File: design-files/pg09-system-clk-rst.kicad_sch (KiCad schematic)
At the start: 16 parts, among them J201 Clock Source, J202 Reset Connector, Q201 2N7000, SW201 SW_Push, U201 CD74ACT109, U202 CD74ACT163, U203 DS1813, X201 ACO-32.000MHz

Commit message: Assign a bunch of footprints.
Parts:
- C201, C202, C203: footprint (none) -> Capacitor_THT:C_Disc_D6.0mm_W4.4mm_P5.00mm
- U201, U202: footprint (none) -> Package_DIP:DIP-16_W7.62mm_Socket
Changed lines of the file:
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@@
       (effects (font (size 1.27 1.27)) (justify left))
     )
-    (property "Footprint" "" (at 196.215 79.375 0)
+    (property "Footprint" "Package_DIP:DIP-16_W7.62mm_Socket" (at 196.215 79.375 0)
       (effects (font (size 1.27 1.27)) hide)
     )
@@
       (effects (font (size 1.27 1.27)) (justify left))
     )
-    (property "Footprint" "" (at 214.63 110.49 0)
+    (property "Footprint" "Capacitor_THT:C_Disc_D6.0mm_W4.4mm_P5.00mm" (at 214.63 110.49 0)
       (effects (font (size 1.27 1.27)) hide)
     )
@@
       (effects (font (size 1.27 1.27)) (justify left))
     )
-    (property "Footprint" "" (at 204.47 110.49 0)
+    (property "Footprint" "Capacitor_THT:C_Disc_D6.0mm_W4.4mm_P5.00mm" (at 204.47 110.49 0)
       (effects (font (size 1.27 1.27)) hide)
     )
@@
       (effects (font (size 1.27 1.27)) (justify left))
     )
-    (property "Footprint" "" (at 194.31 110.49 0)
+    (property "Footprint" "Capacitor_THT:C_Disc_D6.0mm_W4.4mm_P5.00mm" (at 194.31 110.49 0)
       (effects (font (size 1.27 1.27)) hide)
     )
@@
       (effects (font (size 1.27 1.27)) (justify left))
     )
-    (property "Footprint" "" (at 169.545 111.125 0)
+    (property "Footprint" "Package_DIP:DIP-16_W7.62mm_Socket" (at 169.545 111.125 0)
       (effects (font (size 1.27 1.27)) hide)
     )
@@
       (effects (font (size 1.27 1.27)) (justify left))
     )
-    (property "Footprint" "" (at 169.545 79.375 0)
+    (property "Footprint" "Package_DIP:DIP-16_W7.62mm_Socket" (at 169.545 79.375 0)
       (effects (font (size 1.27 1.27)) hide)
     )
@@
       (effects (font (size 1.27 1.27)) (justify left))
     )
-    (property "Footprint" "" (at 95.885 89.535 0)
-      (effects (font (size 1.27 1.27)) hide)
-    )
+    (property "Footprint" "Package_DIP:DIP-16_W7.62mm_Socket" (at 95.885 89.535 0)
+      (effects (font (size 1.27 1.27)) hide)
+    )

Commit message: Finish assigning footprints.
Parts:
- R201, R202, R203, R204, R205: footprint (none) -> Resistor_THT:R_Axial_DIN0207_L6.3mm_D2.5mm_P7.62mm_Horizontal
- SW201: footprint (none) -> Button_Switch_THT:SW_PUSH_6mm
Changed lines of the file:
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@@
       (effects (font (size 1.27 1.27)) (justify left))
     )
-    (property "Footprint" "" (at 220.345 76.835 0)
+    (property "Footprint" "Resistor_THT:R_Axial_DIN0207_L6.3mm_D2.5mm_P7.62mm_Horizontal" (at 220.345 76.835 0)
       (effects (font (size 1.27 1.27)) hide)
     )
@@
       (effects (font (size 1.27 1.27)) (justify right))
     )
-    (property "Footprint" "" (at 212.725 88.265 0)
+    (property "Footprint" "Resistor_THT:R_Axial_DIN0207_L6.3mm_D2.5mm_P7.62mm_Horizontal" (at 212.725 88.265 0)
       (effects (font (size 1.27 1.27)) hide)
     )
@@
       (effects (font (size 1.27 1.27)))
     )
-    (property "Footprint" "" (at 100.965 163.195 0)
+    (property "Footprint" "Button_Switch_THT:SW_PUSH_6mm" (at 100.965 163.195 0)
       (effects (font (size 1.27 1.27)) hide)
     )
@@
       (effects (font (size 1.27 1.27)) (justify right))
     )
-    (property "Footprint" "" (at 84.455 151.765 0)
+    (property "Footprint" "Resistor_THT:R_Axial_DIN0207_L6.3mm_D2.5mm_P7.62mm_Horizontal" (at 84.455 151.765 0)
       (effects (font (size 1.27 1.27)) hide)
     )
@@
       (effects (font (size 1.27 1.27)))
     )
-    (property "Footprint" "" (at 219.075 59.69 0)
+    (property "Footprint" "Resistor_THT:R_Axial_DIN0207_L6.3mm_D2.5mm_P7.62mm_Horizontal" (at 219.075 59.69 0)
       (effects (font (size 1.27 1.27)) hide)
     )
@@
       (effects (font (size 1.27 1.27)))
     )
-    (property "Footprint" "" (at 219.075 66.675 0)
-      (effects (font (size 1.27 1.27)) hide)
-    )
+    (property "Footprint" "Resistor_THT:R_Axial_DIN0207_L6.3mm_D2.5mm_P7.62mm_Horizontal" (at 219.075 66.675 0)
+      (effects (font (size 1.27 1.27)) hide)
+    )

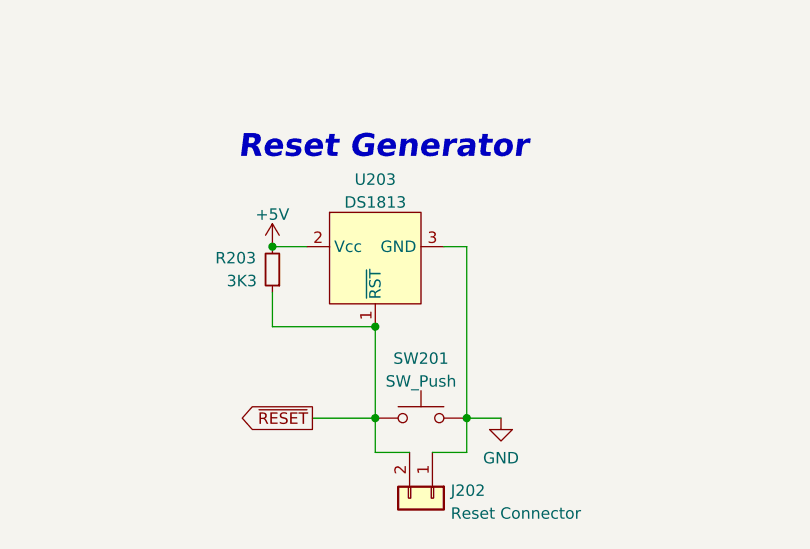
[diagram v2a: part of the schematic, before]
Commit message: Fix various errors and omissions discovered while working on the first cut of the PCB layout.
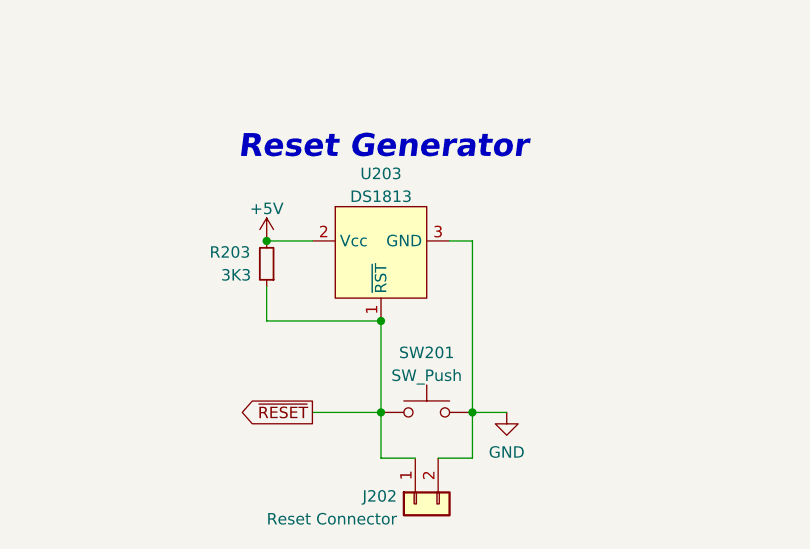
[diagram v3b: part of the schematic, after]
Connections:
- net GND: now also J202.2 (Pin_2); no longer J202.1 (Pin_1)
- net ~{RESET}: now also J202.1 (Pin_1); no longer J202.2 (Pin_2)
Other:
- moved on the sheet: J202, R203, SW201, U203

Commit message: Specify a physically smaller bypass cap.
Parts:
- C201, C202, C203: footprint Capacitor_THT:C_Disc_D6.0mm_W4.4mm_P5.00mm -> Capacitor_THT:C_Disc_D3.8mm_W2.6mm_P2.50mm
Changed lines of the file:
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@@
       (effects (font (size 1.27 1.27)) (justify left))
     )
-    (property "Footprint" "Capacitor_THT:C_Disc_D6.0mm_W4.4mm_P5.00mm" (at 214.63 110.49 0)
+    (property "Footprint" "Capacitor_THT:C_Disc_D3.8mm_W2.6mm_P2.50mm" (at 214.63 110.49 0)
       (effects (font (size 1.27 1.27)) hide)
     )
@@
       (effects (font (size 1.27 1.27)) (justify left))
     )
-    (property "Footprint" "Capacitor_THT:C_Disc_D6.0mm_W4.4mm_P5.00mm" (at 204.47 110.49 0)
+    (property "Footprint" "Capacitor_THT:C_Disc_D3.8mm_W2.6mm_P2.50mm" (at 204.47 110.49 0)
       (effects (font (size 1.27 1.27)) hide)
     )
@@
       (effects (font (size 1.27 1.27)) (justify left))
     )
-    (property "Footprint" "Capacitor_THT:C_Disc_D6.0mm_W4.4mm_P5.00mm" (at 194.31 110.49 0)
-      (effects (font (size 1.27 1.27)) hide)
-    )
+    (property "Footprint" "Capacitor_THT:C_Disc_D3.8mm_W2.6mm_P2.50mm" (at 194.31 110.49 0)
+      (effects (font (size 1.27 1.27)) hide)
+    )
